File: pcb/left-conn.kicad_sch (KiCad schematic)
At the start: 19 parts, among them J3 USB_C_Receptacle, J4 USB_C_Plug

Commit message: Added MPNs and footprints for I think everything.
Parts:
- J3: footprint (none) -> Connector_USB:USB_C_Receptacle_Amphenol_12401548E4-2A; MPN (none) -> 12401548E4#2A
- J4: footprint (none) -> Connector_USB:USB_C_Receptacle_GCT_USB4085; MPN (none) -> USB4085-GF-A
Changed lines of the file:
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@@
 			)
 		)
-		(property "Footprint" ""
+		(property "Footprint" "Connector_USB:USB_C_Receptacle_Amphenol_12401548E4-2A"
 			(at 275.59 181.61 0)
 			(effects
@@
 		)
 		(property "Description" "USB Full-Featured Type-C Receptacle connector"
+			(at 279.4 181.61 0)
+			(effects
+				(font
+					(size 1.27 1.27)
+				)
+				(hide yes)
+			)
+		)
+		(property "MPN" "12401548E4#2A "
 			(at 279.4 181.61 0)
 			(effects
@@
 			)
 		)
-		(property "Footprint" ""
+		(property "Footprint" "Connector_USB:USB_C_Receptacle_GCT_USB4085"
 			(at 275.59 57.15 0)
 			(effects
@@
 			(at 279.4 57.15 0)
 			(effects
+				(font
+					(size 1.27 1.27)
+				)
+				(hide yes)
+			)
+		)
+		(property "MPN" "USB4085-GF-A "
+			(at 279.4 57.15 0)
+			(effects

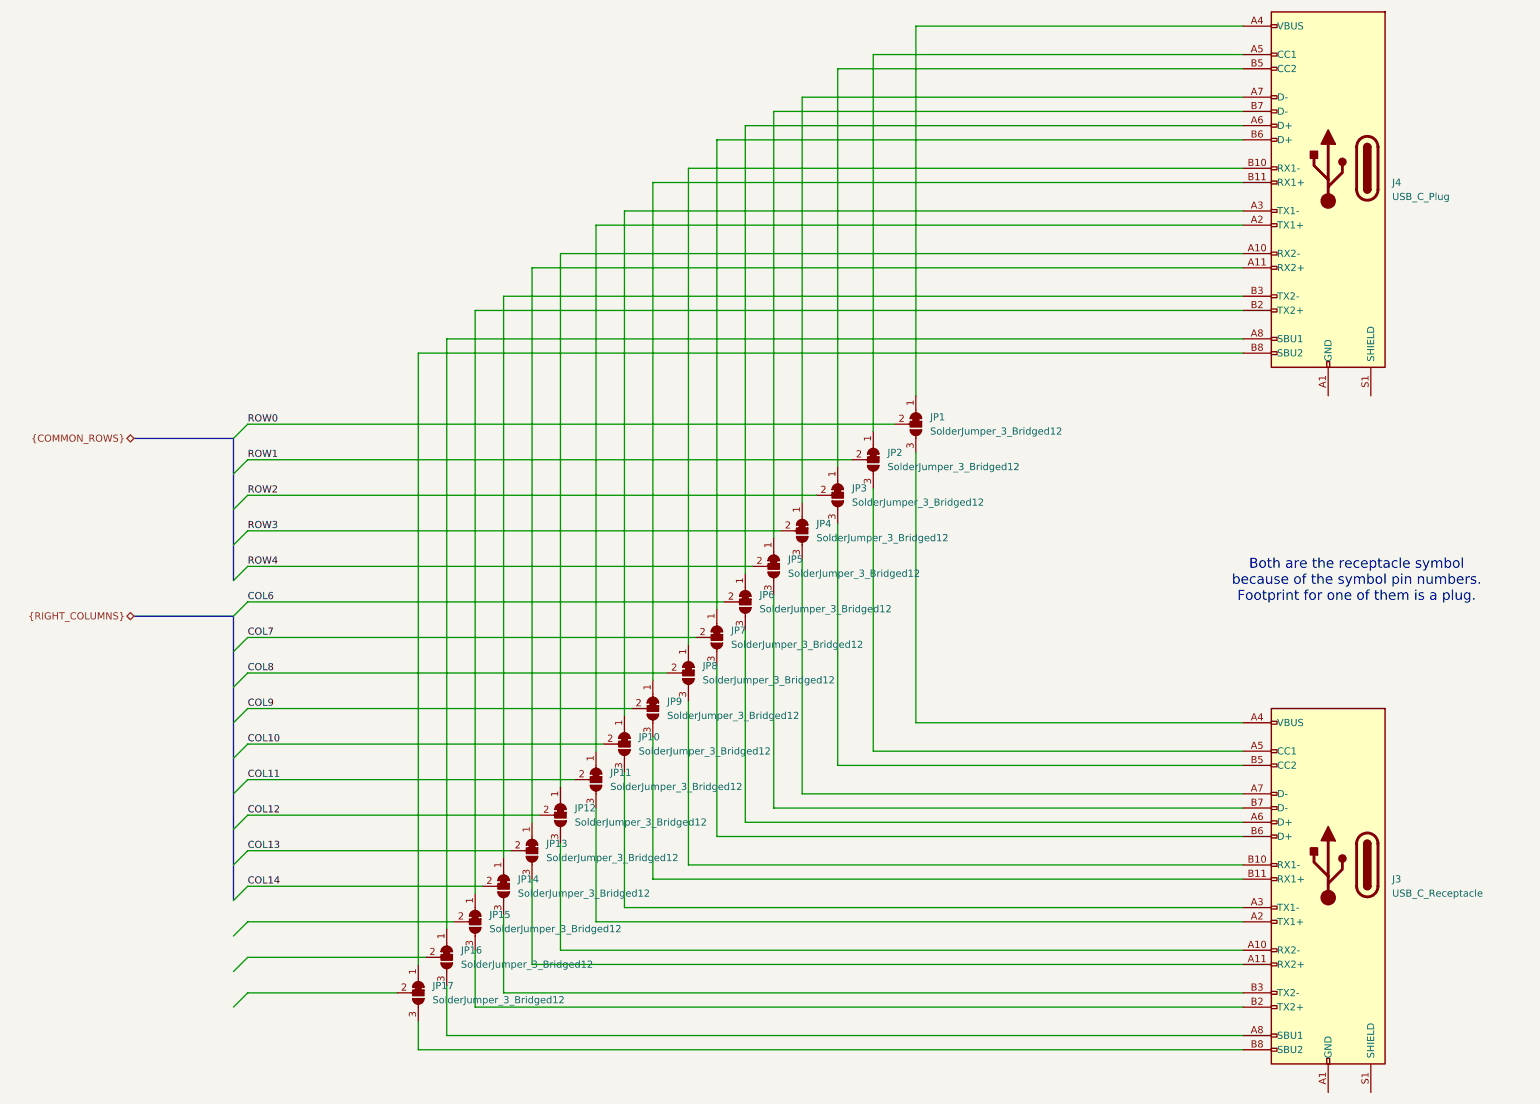
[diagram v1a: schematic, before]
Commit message: Continuing...no one will read this but me.
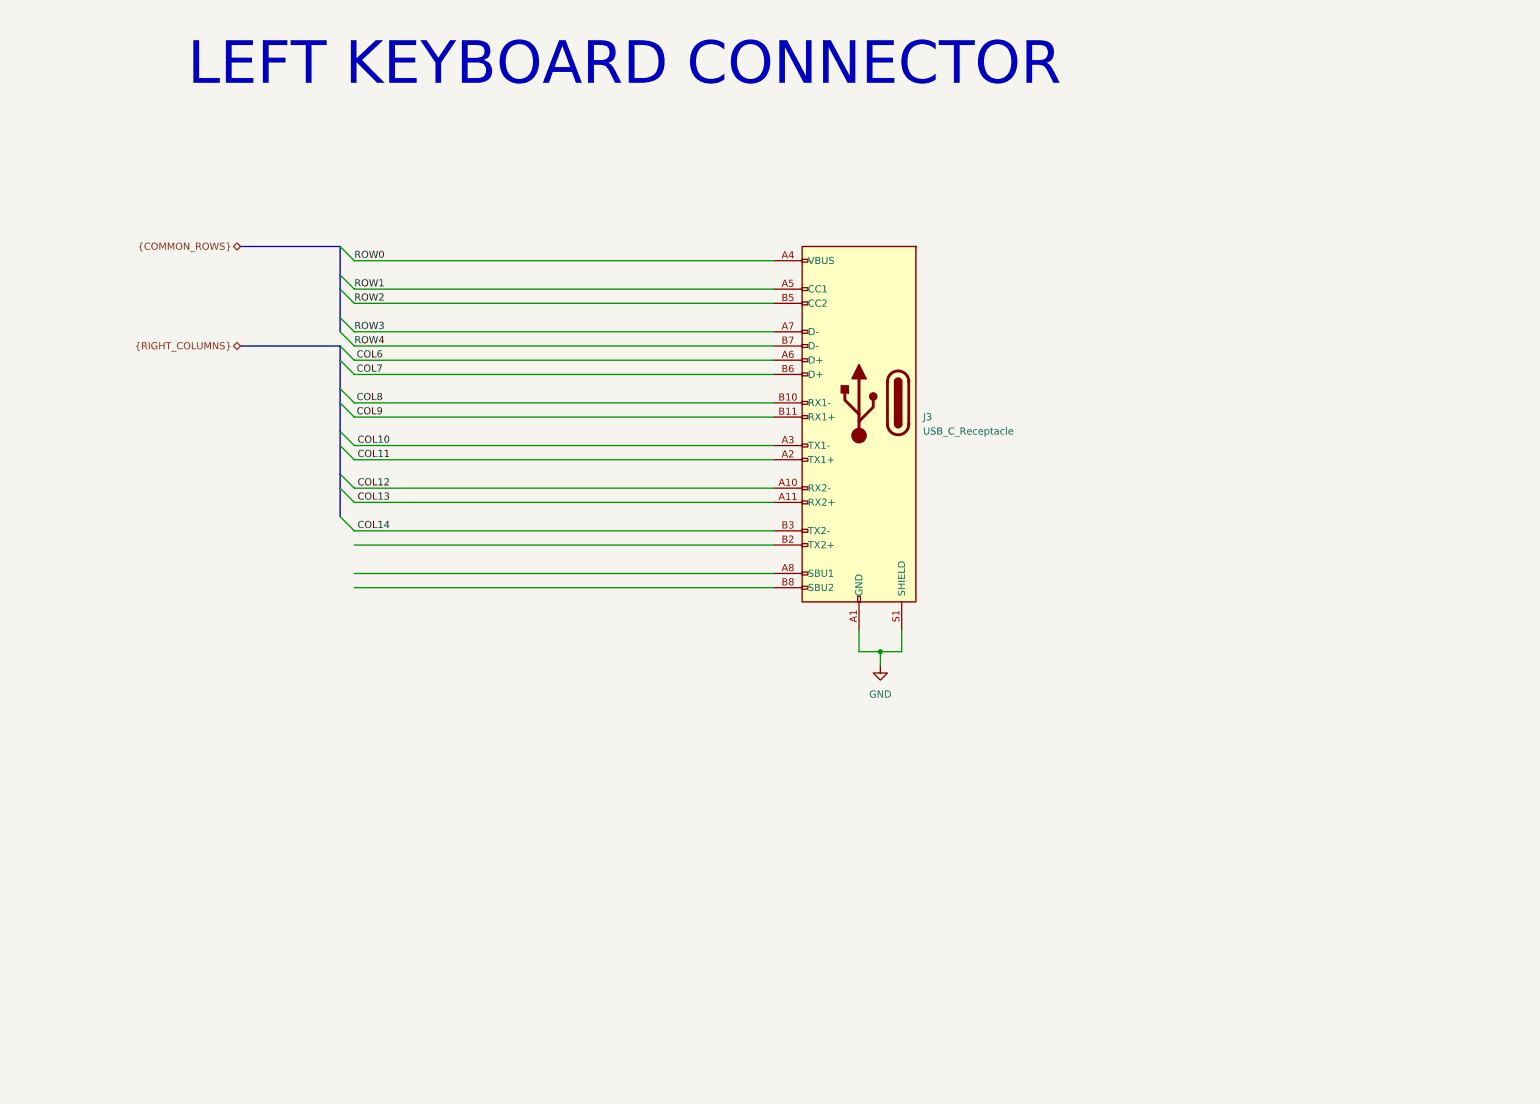
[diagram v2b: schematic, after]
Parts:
- removed J4: USB_C_Plug, Connector_USB:USB_C_Receptacle_GCT_USB4085, symbol Connector:USB_C_Receptacle
- removed JP1, JP10, JP11, JP12, JP13, JP14, JP15, JP16, JP17, JP2, JP3, JP4, JP5, JP6, JP7, JP8, JP9: SolderJumper_3_Bridged12, Jumper:SolderJumper-3_P1.3mm_Bridged12_Pad1.0x1.5mm, symbol Jumper:SolderJumper_3_Bridged12
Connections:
- net COL10: now also J3.A3 (TX1-)
- net COL11: now also J3.A2 (TX1+)
- net COL12: now also J3.A10 (RX2-)
- net COL13: now also J3.A11 (RX2+)
- net COL14: now also J3.B3 (TX2-)
- net COL6: now also J3.A6 (D+)
- net COL7: now also J3.B6 (D+)
- net COL8: now also J3.B10 (RX1-)
- net COL9: now also J3.B11 (RX1+)
- net ROW0: now also J3.A4 (VBUS), J3.A9 (VBUS), J3.B4 (VBUS), J3.B9 (VBUS)
- net ROW1: now also J3.A5 (CC1)
- net ROW2: now also J3.B5 (CC2)
- net ROW3: now also J3.A7 (D-)
- net ROW4: now also J3.B7 (D-)
- net GND: now reaches J3.A1 (GND), J3.A12 (GND), J3.B1 (GND), J3.B12 (GND)
- net GND: now also J3.S1 (SHIELD)
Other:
- note added: "LEFT KEYBOARD CONNECTOR"
- note removed: "Both are the receptacle symbol because of the symbol pin numbers. Footprint for one of them is a plug."
- moved on the sheet: J3
